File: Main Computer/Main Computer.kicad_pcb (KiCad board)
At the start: 2 copper layers, 56 x 65 mm, 11 parts, among them J1 Pi 5 GPIO HEADER, J3 Conn_01x02, J4 CAN to outer connector, U1 RFM9X Breakout

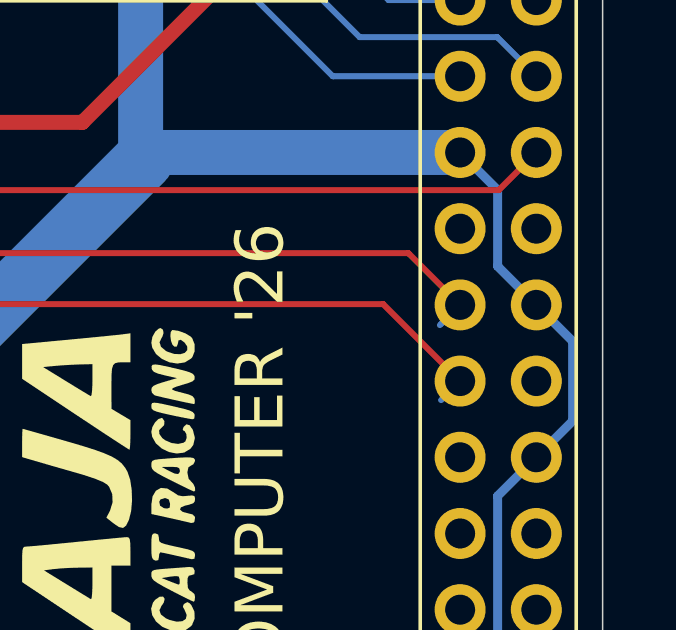
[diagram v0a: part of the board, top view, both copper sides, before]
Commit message: update stuff, fix error
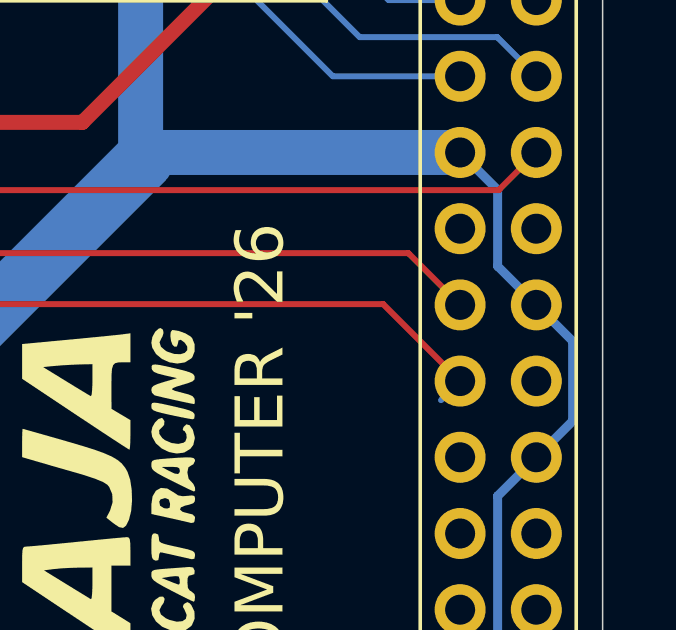
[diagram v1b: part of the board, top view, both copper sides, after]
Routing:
- net RADIO_INT: track 29.8 -> 28.8 mm
